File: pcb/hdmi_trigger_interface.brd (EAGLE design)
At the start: 78.7 x 63.5 mm, 41 parts, among them P1 10029449-001RLF, P2 10029449-001RLF, U1 TPD12S016PWR, U2 TPD12S016PWR

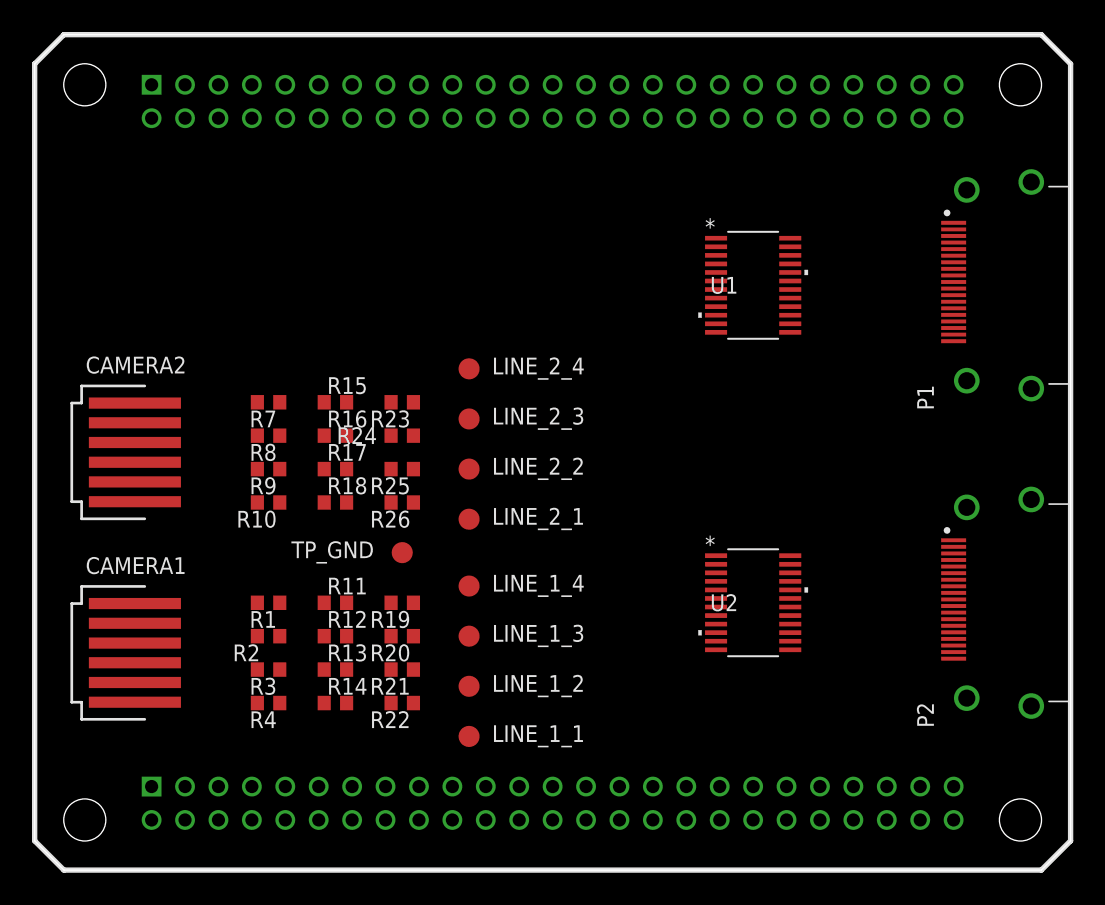
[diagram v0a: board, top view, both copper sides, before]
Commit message: almost done with routing
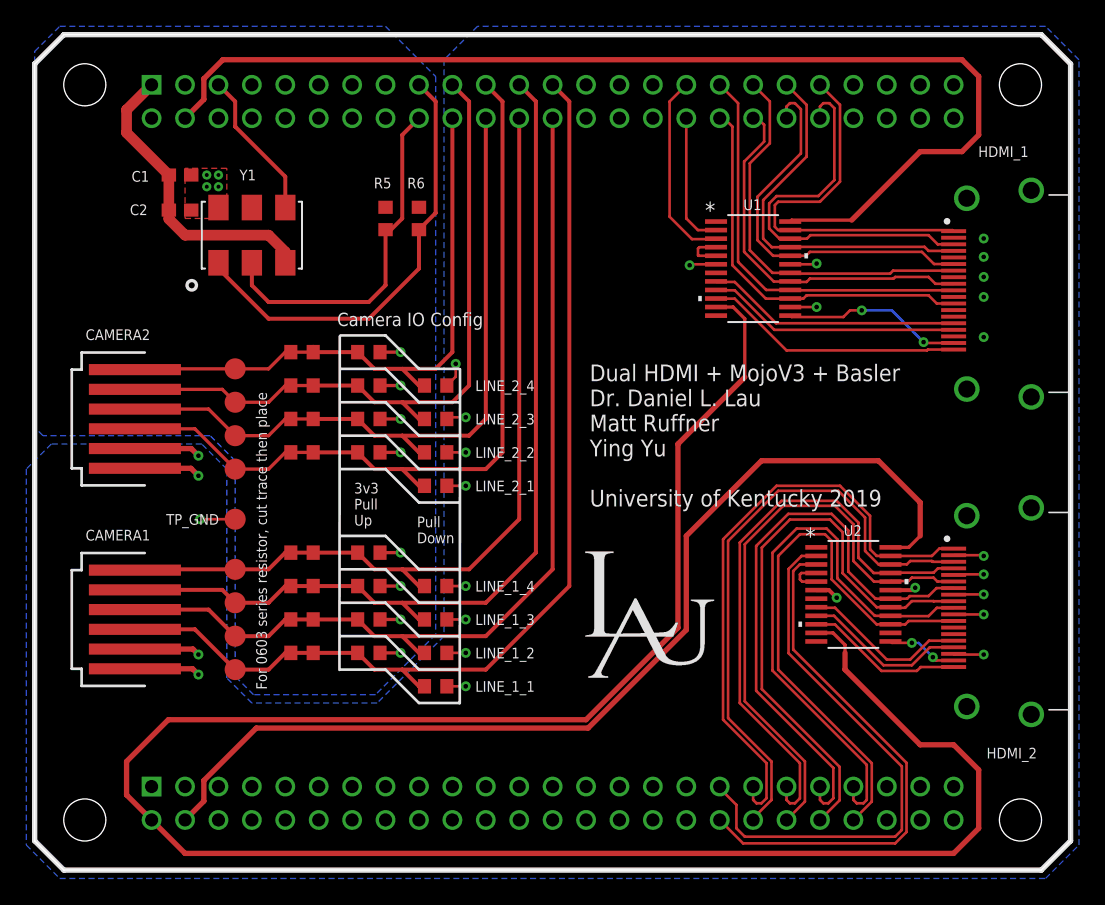
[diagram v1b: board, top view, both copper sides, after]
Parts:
- removed P1, P2: 10029449-001RLF, 10029449-001RLF:FCI_10029449-001RLF
- added C1: 0.1uF, rcl:C0603
- added C2: 1uF, rcl:C0603
- added HDMI_1, HDMI_2: 10029449-001RLF, 10029449-001RLF:FCI_10029449-001RLF
- added R5, R6: 3k, rcl:R0603
- added Y1: SI514, lupa300-components:XTAL-6PIN
- moved LINE_1_1 18.5 mm to (15.2, 15.2)
- moved LINE_1_2 18.2 mm to (15.2, 17.8)
- moved LINE_2_1 18.2 mm to (15.2, 30.5)
- moved LINE_1_3 18.0 mm to (15.2, 20.3)
- moved LINE_2_2 18.0 mm to (15.2, 33.0)
- moved LINE_1_4 17.8 mm to (15.2, 22.9)
- moved LINE_2_3 17.8 mm to (15.2, 35.6)
- moved LINE_2_4 17.8 mm to (15.2, 38.1)
- moved TP_GND 13.0 mm to (15.2, 26.7)
- moved U2 7.65 mm to (62.2, 21.0)
- moved R14 4.58 mm to (25.4, 16.5)
- moved R4 4.58 mm to (20.3, 16.5)
- moved R13 4.58 mm to (25.4, 19.1)
- moved R3 4.58 mm to (20.3, 19.1)
- moved R1 4.58 mm to (20.3, 24.1)
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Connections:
- removed net GND@1: U$1.GND@1, U$1.GND@2, U$1.GND@3, U$1.GND@4
- removed net GND_2: U1.6, U2.6
- removed net GND_3: U2.14
- removed net N$1: U1.13
- removed net N$14: U1.19
- removed net N$19: U1.14
- removed net N$22: P1.18
- removed net N$3: U1.24
- removed net N$39: P2.18
- removed net VCC5V: U1.11, U2.11
- removed net VCCA: U2.24
- new net 5V: U$1.RAW@1, U$1.RAW@2, U1.11, U2.11
- new net 5VHDMI1: HDMI_1.18, U1.13
- new net 5VHDMI2: HDMI_2.18, U2.13
- new net CTHPD1: U1.12
- new net CTHPD2: U2.12
- new net HP1_M: U1.4, U1.5
- new net HP2_M: U2.4, U2.5
- new net PROG_CLK: U$1.51, Y1.P$4
- new net SCL2_M: U$1.112, U2.2
- new net SCL_C: R5.1, U$1.23, Y1.P$2
- new net SDA2_M: U$1.111, U2.3
- new net SDA_C: R6.1, U$1.24, Y1.P$1
- net 3V3: now also C1.1, C2.1, R5.2, R6.2, U1.24, U2.24, Y1.P$6
- net CLK1_N: now also HDMI_1.12; no longer P1.12
- net CLK1_P: now also HDMI_1.10; no longer P1.10
- net CLK2_N: now also HDMI_2.12, U2.15; no longer P2.12
- net CLK2_P: now also HDMI_2.10, U2.16; no longer P2.10
- net D01_N: now also HDMI_1.9; no longer P1.9
- net D01_P: now also HDMI_1.7; no longer P1.7
- net D02_N: now also HDMI_2.9, U2.17; no longer P2.9
- net D02_P: now also HDMI_2.7, U2.18; no longer P2.7
- net D11_N: now also HDMI_1.6; no longer P1.6
- net D11_P: now also HDMI_1.4; no longer P1.4
- net D12_N: now also HDMI_2.6, U2.20; no longer P2.6
- net D12_P: now also HDMI_2.4, U2.21; no longer P2.4
- net D21_N: now also HDMI_1.3; no longer P1.3
- net D21_P: now also HDMI_1.1; no longer P1.1
- net D22_N: now also HDMI_2.3, U2.22; no longer P2.3
- net D22_P: now also HDMI_2.1, U2.23; no longer P2.1
- net GND: now also C1.2, C2.2, HDMI_1.11, HDMI_1.17, HDMI_1.2, HDMI_1.5, HDMI_1.8, HDMI_2.11, HDMI_2.17, HDMI_2.2, HDMI_2.5, HDMI_2.8, U$1.GND@1, U$1.GND@2, U$1.GND@3, U$1.GND@4, U$1.GND@6, U1.14, U1.19, U1.6, U2.14, U2.6, Y1.P$3; no longer P1.11, P1.17, P1.2, P1.5, P1.8, P2.11, P2.17, P2.2, P2.5, P2.8
- net HP1: now also HDMI_1.19; no longer P1.19
- net HP2: now also HDMI_2.19, U2.10; no longer P2.19
- net LINE_1_1: now also U$1.12; no longer LINE_1_1.TP
- net LINE_1_2: now also U$1.11; no longer LINE_1_2.TP
- net LINE_1_3: now also U$1.15; no longer LINE_1_3.TP
- net LINE_1_4: now also U$1.14; no longer LINE_1_4.TP
- net LINE_2_1: now also U$1.17; no longer LINE_2_1.TP
- net LINE_2_2: now also U$1.16; no longer LINE_2_2.TP
- net LINE_2_3: now also U$1.22; no longer LINE_2_3.TP
- net LINE_2_4: now also U$1.21; no longer LINE_2_4.TP
- net N$10: now also LINE_2_3.TP
- net N$11: now also LINE_2_2.TP
- net N$12: now also LINE_2_1.TP
- net N$5: now also LINE_1_4.TP
- net N$6: now also LINE_1_3.TP
- net N$7: now also LINE_1_2.TP
- net N$8: now also LINE_1_1.TP
- net N$9: now also LINE_2_4.TP
- net SCL1: now also HDMI_1.15; no longer P1.15
- net SCL2: now also HDMI_2.15, U2.8; no longer P2.15, U$1.112
- net SDA1: now also HDMI_1.16; no longer P1.16
- net SDA2: now also HDMI_2.16, U2.9; no longer P2.16, U$1.111
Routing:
- net 3V3: track 0.00 -> 176.4 mm, vias 0 -> 12
- net 5V: track 0.00 -> 166.4 mm
- net GND: track 0.00 -> 79.2 mm, vias 0 -> 23
- net LINE_1_1: track 0.00 -> 63.5 mm
- net LINE_1_3: track 0.00 -> 57.3 mm
- net LINE_1_2: track 0.00 -> 57.3 mm
- net LINE_1_4: track 0.00 -> 50.5 mm
- net D22_P: track 0.00 -> 46.5 mm
- net LINE_2_1: track 0.00 -> 46.1 mm
- net D22_N: track 0.00 -> 45.8 mm
- net D12_P: track 0.00 -> 45.2 mm
- net D12_N: track 0.00 -> 44.8 mm
- net D02_P: track 0.00 -> 44.8 mm
- net D02_N: track 0.00 -> 44.0 mm
- net CLK2_P: track 0.00 -> 43.3 mm
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- added copper zone on layer 1, net 3V3
- added copper zone on layer 16, net 3V3
- added copper zone on layer 16, net GND
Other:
- board text added: "3v3 Pull Up"
- board text added: "Camera IO Config"
- board text added: "Dual HDMI + MojoV3 + Basler Dr. Daniel L. Lau Matt Ruffner Ying Yu University of Kentucky 2019"
- board text added: "For 0603 series resistor, cut trace then place"
- board text added: "Pull Down"
